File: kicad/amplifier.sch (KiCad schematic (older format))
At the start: 21 parts, among them U6 GS8332-SR

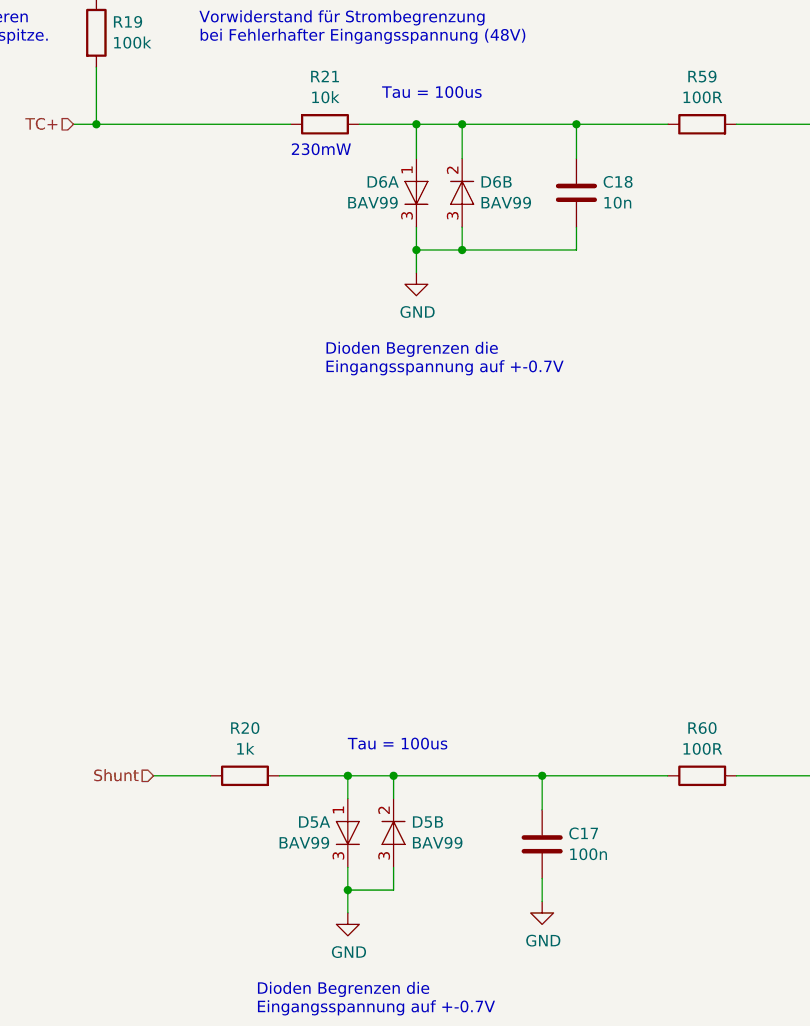
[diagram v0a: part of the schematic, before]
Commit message: Neu: Spannungsreferenz TL431, Laout Fertig, TODO: Labels
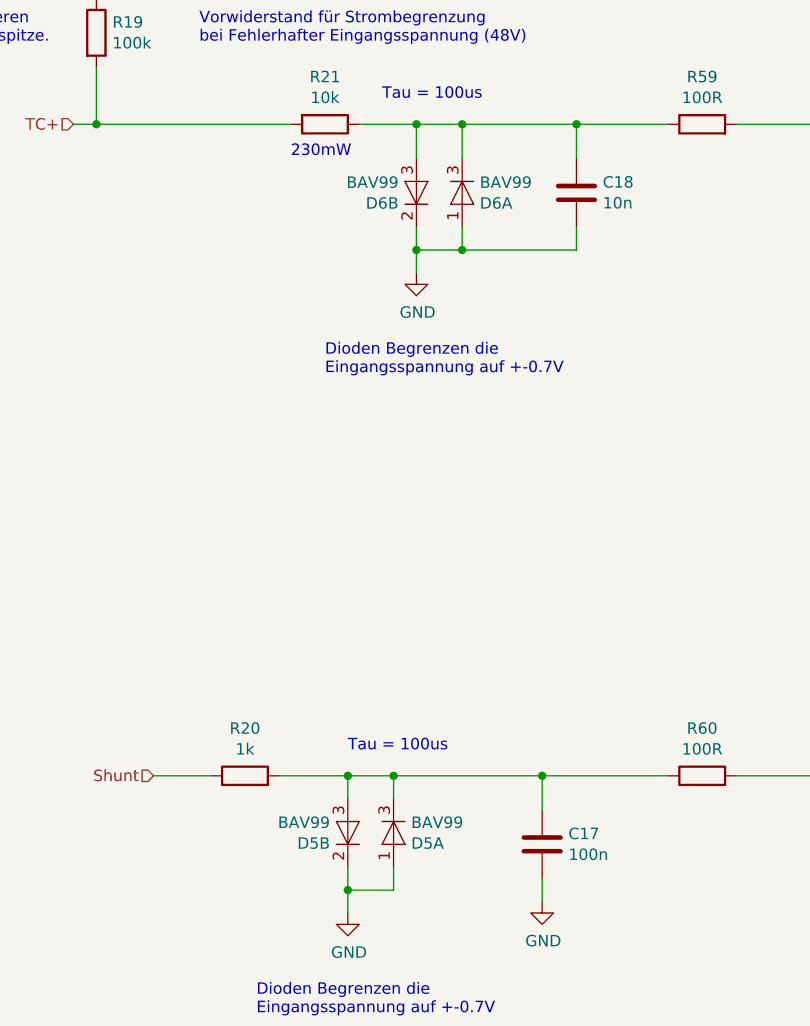
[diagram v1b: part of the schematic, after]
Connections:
- net GND: now also D5.1 (A), D5.2 (K), D6.1 (A), D6.2 (K); no longer D5.3 (A), D5.3 (K), D6.3 (A), D6.3 (K)
- net at C18.1, R21.1, R59.1: now also D6.3 (A), D6.3 (K); no longer D6.1 (A), D6.2 (K)
- net at C17.2, R20.2, R60.1: now also D5.3 (A), D5.3 (K); no longer D5.1 (A), D5.2 (K)
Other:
- moved on the sheet: D5A, D5B, D6A, D6B
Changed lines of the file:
@@
 L jbc-miniregler-rescue:BAV99-Diode D6
 U 2 1 608F0A12
+P 3550 2700
+F 0 "D6" V 3504 2778 50  0000 L CNN
+F 1 "BAV99" V 3595 2778 50  0000 L CNN
+F 2 "Package_TO_SOT_SMD:SOT-23" H 3550 2550 50  0001 C CNN
+F 3 "https://assets.nexperia.com/documents/data-sheet/BAV99_SER.pdf" H 3550 2800 50  0001 C CNN
+F 4 "C181111" H 3550 2700 50  0001 C CNN "DistOrderNr"
+F 5 "LCSC" H 3550 2700 50  0001 C CNN "Distributor"
+F 6 "BAV99" H 3550 2700 50  0001 C CNN "ManPartNr"
+F 7 "Guangdong Hottech" H 3550 2700 50  0001 C CNN "Manufacturer"
+F 8 "70V 200mA 1.25V @ 150mA 6ns SOT-23 Switching Diode" H 3550 2700 50  0001 C CNN "Notes"
+F 9 "0.0073" H 3550 2700 50  0001 C CNN "PriceEUR"
+F 10 "500" H 3550 2700 50  0001 C CNN "PriceForQty"
+F 11 "https://lcsc.com/product-detail/Switching-Diode_BAV99-chip0-23_C181111.html" H 3550 2700 50  0001 C CNN "Weblink"
+	2    3550 2700
+	0    -1   -1   0
+$EndComp
+$Comp
+L jbc-miniregler-rescue:BAV99-Diode D6
+U 1 1 608F1916
 P 3750 2700
-F 0 "D6" V 3704 2778 50  0000 L CNN
-F 1 "BAV99" V 3795 2778 50  0000 L CNN
+F 0 "D6" V 3796 2777 50  0000 L CNN
+F 1 "BAV99" V 3705 2777 50  0000 L CNN
 F 2 "Package_TO_SOT_SMD:SOT-23" H 3750 2550 50  0001 C CNN
 F 3 "https://assets.nexperia.com/documents/data-sheet/BAV99_SER.pdf" H 3750 2800 50  0001 C CNN
@@
 F 10 "500" H 3750 2700 50  0001 C CNN "PriceForQty"
 F 11 "https://lcsc.com/product-detail/Switching-Diode_BAV99-chip0-23_C181111.html" H 3750 2700 50  0001 C CNN "Weblink"
-	2    3750 2700
+	1    3750 2700
 	0    1    1    0
-$EndComp
-$Comp
-L jbc-miniregler-rescue:BAV99-Diode D6
-U 1 1 608F1916
-P 3550 2700
-F 0 "D6" V 3596 2777 50  0000 L CNN
-F 1 "BAV99" V 3505 2777 50  0000 L CNN
-F 2 "Package_TO_SOT_SMD:SOT-23" H 3550 2550 50  0001 C CNN
-F 3 "https://assets.nexperia.com/documents/data-sheet/BAV99_SER.pdf" H 3550 2800 50  0001 C CNN
-F 4 "C181111" H 3550 2700 50  0001 C CNN "DistOrderNr"
-F 5 "LCSC" H 3550 2700 50  0001 C CNN "Distributor"
-F 6 "BAV99" H 3550 2700 50  0001 C CNN "ManPartNr"
-F 7 "Guangdong Hottech" H 3550 2700 50  0001 C CNN "Manufacturer"
-F 8 "70V 200mA 1.25V @ 150mA 6ns SOT-23 Switching Diode" H 3550 2700 50  0001 C CNN "Notes"
-F 9 "0.0073" H 3550 2700 50  0001 C CNN "PriceEUR"
-F 10 "500" H 3550 2700 50  0001 C CNN "PriceForQty"
-F 11 "https://lcsc.com/product-detail/Switching-Diode_BAV99-chip0-23_C181111.html" H 3550 2700 50  0001 C CNN "Weblink"
-	1    3550 2700
-	0    -1   -1   0
 $EndComp
 Wire Wire Line
@@
 L jbc-miniregler-rescue:BAV99-Diode D5
 U 1 1 60B76F32
+P 3450 5500
+F 0 "D5" V 3496 5577 50  0000 L CNN
+F 1 "BAV99" V 3405 5577 50  0000 L CNN
+F 2 "Package_TO_SOT_SMD:SOT-23" H 3450 5350 50  0001 C CNN
+F 3 "https://assets.nexperia.com/documents/data-sheet/BAV99_SER.pdf" H 3450 5600 50  0001 C CNN
+F 4 "C181111" H 3450 5500 50  0001 C CNN "DistOrderNr"
+F 5 "LCSC" H 3450 5500 50  0001 C CNN "Distributor"
+F 6 "BAV99" H 3450 5500 50  0001 C CNN "ManPartNr"
+F 7 "Guangdong Hottech" H 3450 5500 50  0001 C CNN "Manufacturer"
+F 8 "70V 200mA 1.25V @ 150mA 6ns SOT-23 Switching Diode" H 3450 5500 50  0001 C CNN "Notes"
+F 9 "0.0073" H 3450 5500 50  0001 C CNN "PriceEUR"
+F 10 "500" H 3450 5500 50  0001 C CNN "PriceForQty"
+F 11 "https://lcsc.com/product-detail/Switching-Diode_BAV99-chip0-23_C181111.html" H 3450 5500 50  0001 C CNN "Weblink"
+	1    3450 5500
+	0    1    1    0
+$EndComp
+$Comp
+L jbc-miniregler-rescue:BAV99-Diode D5
+U 2 1 60B76F24
 P 3250 5500
-F 0 "D5" V 3296 5577 50  0000 L CNN
-F 1 "BAV99" V 3205 5577 50  0000 L CNN
+F 0 "D5" V 3204 5578 50  0000 L CNN
+F 1 "BAV99" V 3295 5578 50  0000 L CNN
 F 2 "Package_TO_SOT_SMD:SOT-23" H 3250 5350 50  0001 C CNN
 F 3 "https://assets.nexperia.com/documents/data-sheet/BAV99_SER.pdf" H 3250 5600 50  0001 C CNN
@@
 F 10 "500" H 3250 5500 50  0001 C CNN "PriceForQty"
 F 11 "https://lcsc.com/product-detail/Switching-Diode_BAV99-chip0-23_C181111.html" H 3250 5500 50  0001 C CNN "Weblink"
-	1    3250 5500
+	2    3250 5500
 	0    -1   -1   0
 $EndComp
-$Comp
-L jbc-miniregler-rescue:BAV99-Diode D5
-U 2 1 60B76F24
-P 3450 5500
-F 0 "D5" V 3404 5578 50  0000 L CNN
-F 1 "BAV99" V 3495 5578 50  0000 L CNN
-F 2 "Package_TO_SOT_SMD:SOT-23" H 3450 5350 50  0001 C CNN
-F 3 "https://assets.nexperia.com/documents/data-sheet/BAV99_SER.pdf" H 3450 5600 50  0001 C CNN
-F 4 "C181111" H 3450 5500 50  0001 C CNN "DistOrderNr"
-F 5 "LCSC" H 3450 5500 50  0001 C CNN "Distributor"
-F 6 "BAV99" H 3450 5500 50  0001 C CNN "ManPartNr"
-F 7 "Guangdong Hottech" H 3450 5500 50  0001 C CNN "Manufacturer"
-F 8 "70V 200mA 1.25V @ 150mA 6ns SOT-23 Switching Diode" H 3450 5500 50  0001 C CNN "Notes"
-F 9 "0.0073" H 3450 5500 50  0001 C CNN "PriceEUR"
-F 10 "500" H 3450 5500 50  0001 C CNN "PriceForQty"
-F 11 "https://lcsc.com/product-detail/Switching-Diode_BAV99-chip0-23_C181111.html" H 3450 5500 50  0001 C CNN "Weblink"
-	2    3450 5500
-	0    1    1    0
-$EndComp
-Wire Wire Line
+Wire Wire Line
